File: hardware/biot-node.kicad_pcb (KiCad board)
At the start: 2 copper layers, 54.1 x 43.7 mm, 15 parts, among them J1 Test Points, J2 MPU9250 connection, J3 on/off, J4 ATMEL-CORTEX, P1 FTDI/Serial, SW1 SW_Reset, U1 ATSAMR21B18-MZ210PA, U2 LP2985-3.3

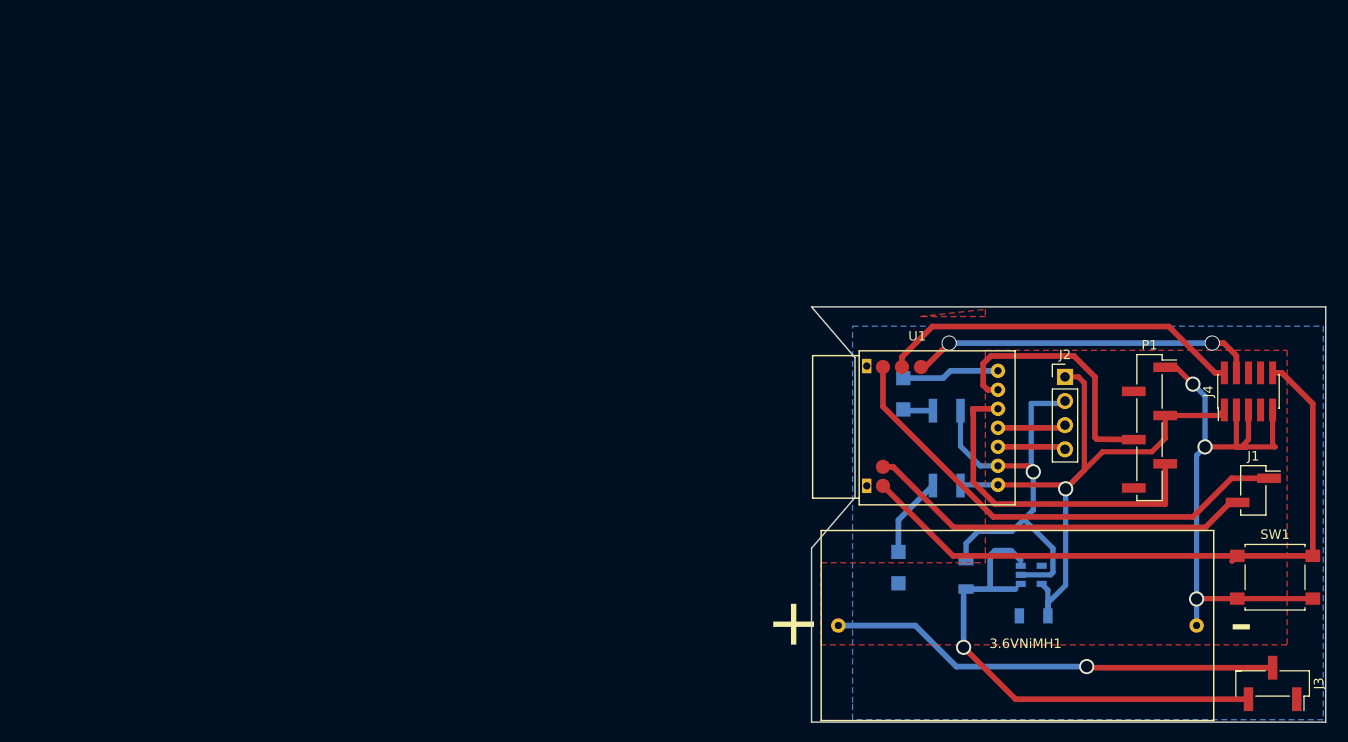
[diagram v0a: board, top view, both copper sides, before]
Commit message: Newer node hardware construction.
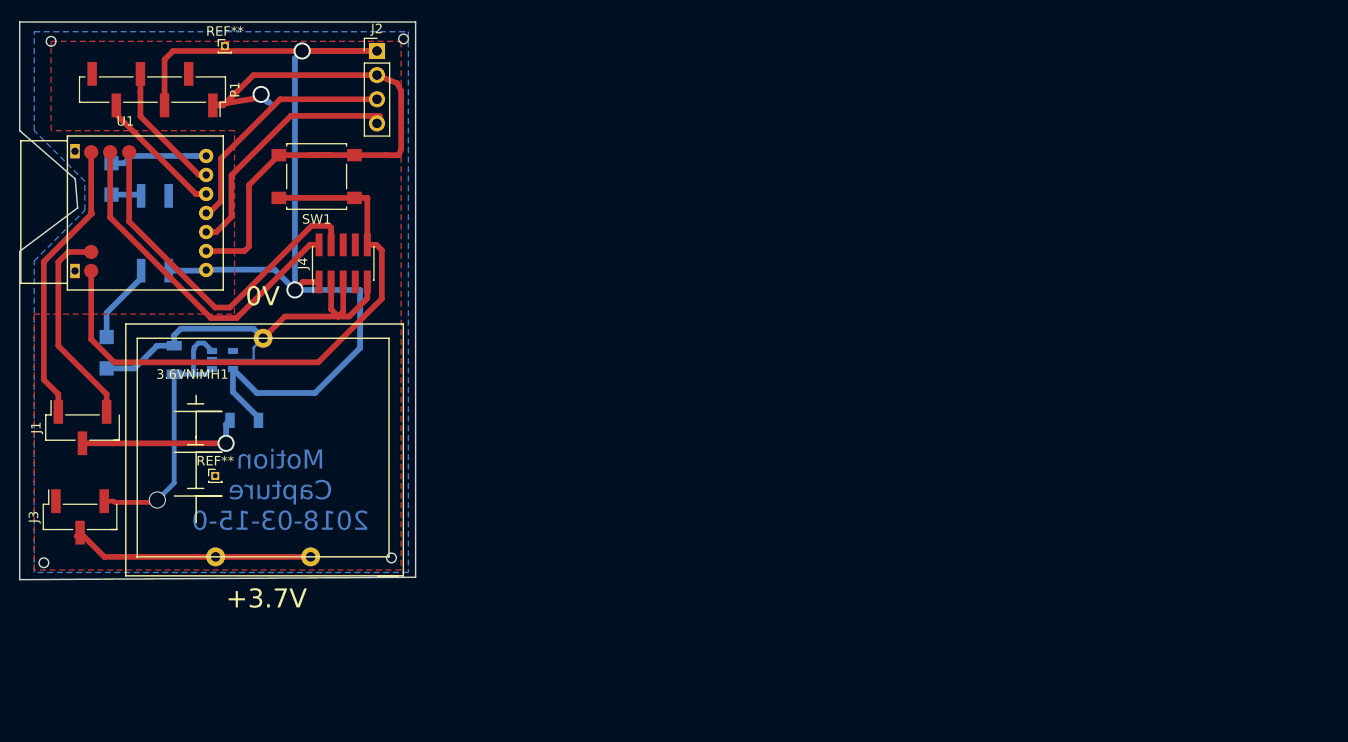
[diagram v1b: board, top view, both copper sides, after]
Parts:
- added REF**: Pin_Header_Straight_1x01_Pitch1.00mm, Pin_Headers:Pin_Header_Straight_1x01_Pitch1.00mm, F.Cu at (132.3, 99.1)
- added REF**: Pin_Header_Straight_1x01_Pitch1.00mm, Pin_Headers:Pin_Header_Straight_1x01_Pitch1.00mm, F.Cu at (133.3, 53.8)
- 3.6VNiMH1: footprint atsamr21:CR123_Battery_Holder -> atsamr21:varta3v200h
- D1: value SIGNAL -> 20mA
- D2: value PWR -> 20mA
- J1: value Test Points -> test points; footprint Pin_Headers:Pin_Header_Straight_1x02_Pitch2.54mm_SMD_Pin1Right -> Pin_Headers:Pin_Header_Straight_1x03_Pitch2.54mm_SMD_Pin1Right
- R1, R2: value 39 -> 68
- moved J3 126.7 mm to (118.1, 103.4), turned to 90 degrees
- moved J1 123.4 mm to (118.4, 94.0), turned to 90 degrees
- moved P1 110.8 mm to (125.7, 58.4), turned to 270 degrees
- moved SW1 109.3 mm to (143.0, 67.6), turned to 180 degrees
- moved J4 96.2 mm to (145.8, 76.7)
- moved U2 88.0 mm to (133.1, 86.9)
- moved C1 86.3 mm to (128.0, 86.9)
- moved D2 86.3 mm to (120.9, 86.1)
- moved R1 86.3 mm to (126.0, 69.6)
- moved R2 86.3 mm to (126.0, 77.5)
- moved U1 86.3 mm to (112.8, 79.5)
- moved D1 86.3 mm to (121.4, 67.8)
- moved C2 85.6 mm to (135.4, 93.2)
- moved J2 80.1 mm to (149.4, 54.4)
- moved 3.6VNiMH1 54.6 mm to (150.6, 84.6), turned to 180 degrees
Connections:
- J1 pad 2: PA15 -> GND
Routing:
- net +3V3: track 65.1 -> 113.9 mm, vias 1 -> 2
- net RX: track 36.3 -> 13.9 mm
- net Net-(3.6VNiMH1-Pad1): track 47.8 -> 25.9 mm, vias 1 -> 0
- net GND: track 111.7 -> 133.5 mm, vias 4 -> 2
- net PA14: track 51.3 -> 30.1 mm
- net Net-(C1-Pad1): track 52.6 -> 32.4 mm
- net SDA: track 7.16 -> 27.0 mm
- net PA15: track 41.0 -> 21.8 mm
- net SCLK: track 7.17 -> 25.7 mm
- net TX: track 27.6 -> 13.9 mm
- net NRST: track 70.6 -> 62.7 mm
- net SWDIO: track 38.3 -> 36.4 mm
- net SWDCLK: track 36.6 -> 37.7 mm, vias 2 -> 0
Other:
- board size 54.1 x 43.7 mm -> 41.7 x 58.7 mm
- net class Default: clearance 0.2 -> 0.15
- net class cnc: via_dia 1.6 -> 1.8
- net class cnc-narrow: clearance 0.3 -> 0.2; via_dia 1.6 -> 1.8; via_drill 1.2 -> 1.4
- rule trace_clearance: 0.2 -> 0.15
- board text added: "Motion Capture 2018-03-15-0"
